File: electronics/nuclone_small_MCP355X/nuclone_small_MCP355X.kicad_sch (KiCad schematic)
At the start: 65 parts, among them J3 nuclone_small_left, J4 nuclone_small_right, J5 FTDI_PINS_1X06, J6 DevBoardUartInput, U1 MCP355X-E_SN

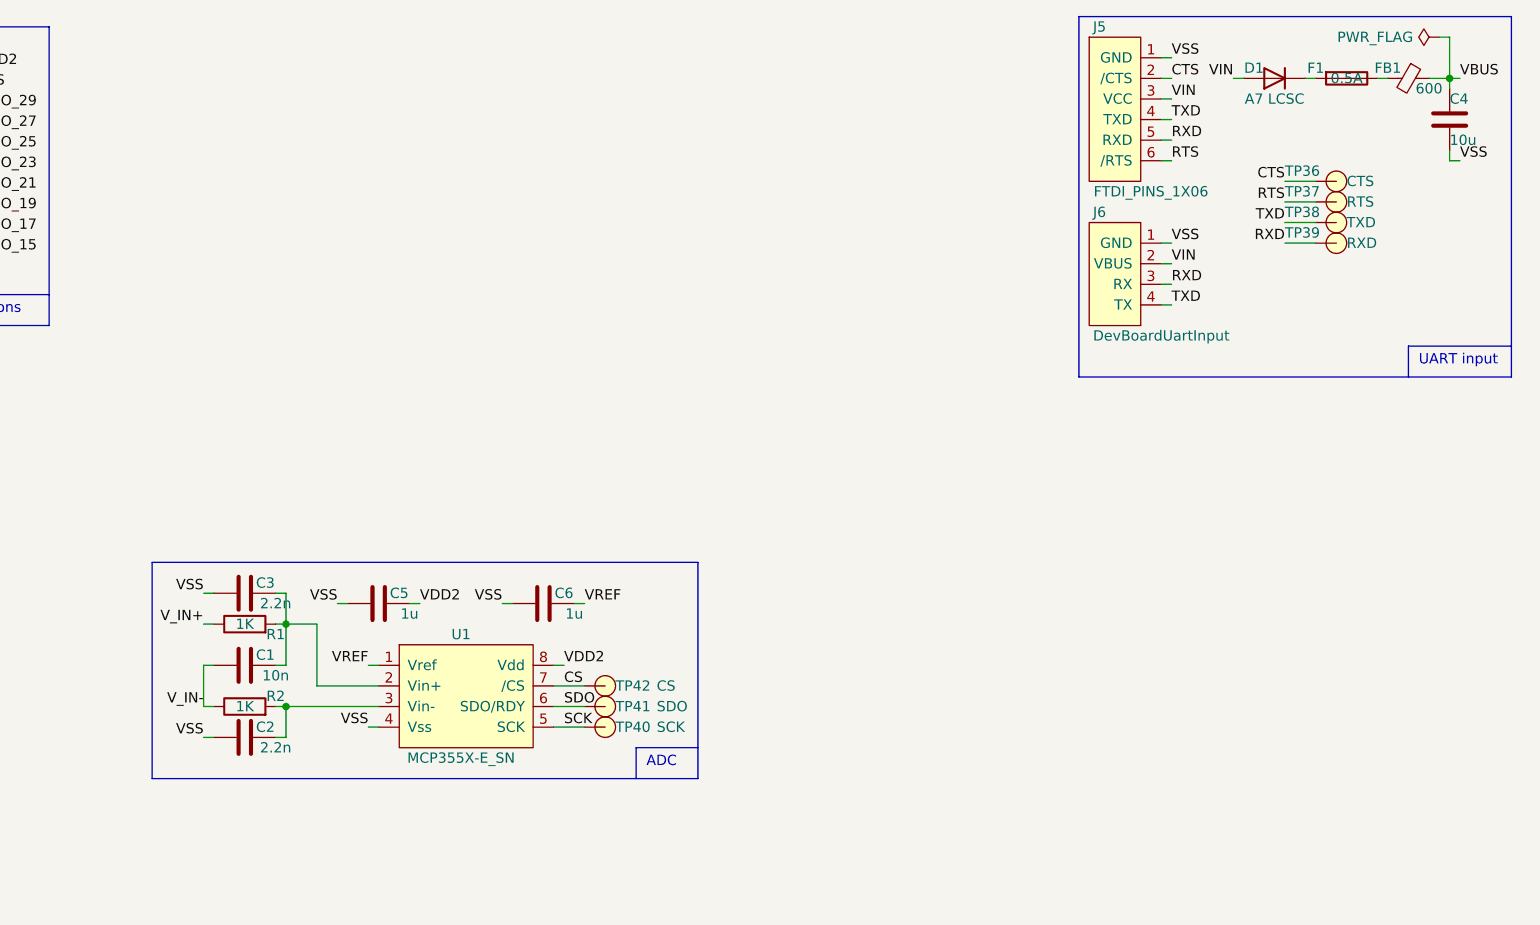
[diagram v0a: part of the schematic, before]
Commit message: WIP schematic definition of MCP355X evaluator
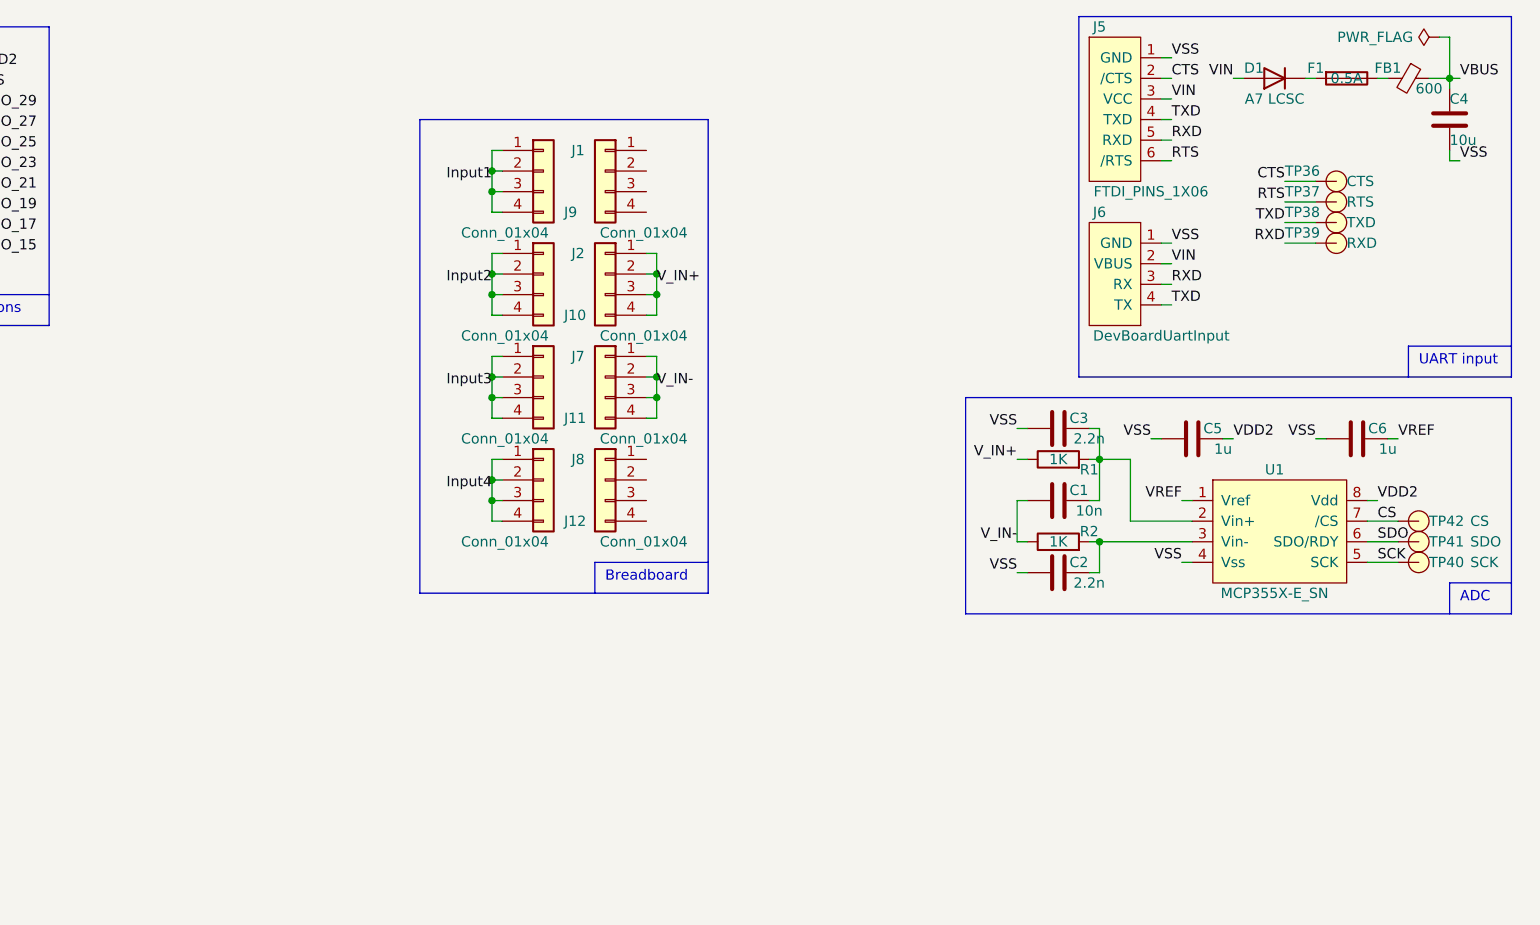
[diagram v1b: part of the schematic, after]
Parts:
- added J1, J10, J11, J12, J2, J7, J8, J9: Conn_01x04, SquantorConnectors:Header-0254-1X04-H010, symbol Connector_Generic:Conn_01x04
- U1: footprint (none) -> SquantorIC:SOIC-8
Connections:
- net V_IN+: now also J2.1 (Pin_1), J2.2 (Pin_2), J2.3 (Pin_3), J2.4 (Pin_4)
- net V_IN-: now also J7.1 (Pin_1), J7.2 (Pin_2), J7.3 (Pin_3), J7.4 (Pin_4)
- new net Input1: J9.1 (Pin_1), J9.2 (Pin_2), J9.3 (Pin_3), J9.4 (Pin_4)
- new net Input2: J10.1 (Pin_1), J10.2 (Pin_2), J10.3 (Pin_3), J10.4 (Pin_4)
- new net Input3: J11.1 (Pin_1), J11.2 (Pin_2), J11.3 (Pin_3), J11.4 (Pin_4)
- new net Input4: J12.1 (Pin_1), J12.2 (Pin_2), J12.3 (Pin_3), J12.4 (Pin_4)
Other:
- note added: "Breadboard"
- moved on the sheet: C1, C2, C3, C5, C6, R1, R2, TP40, TP41, TP42, U1
